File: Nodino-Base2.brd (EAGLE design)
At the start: 64.8 x 27.9 mm, 6 parts, among them CON1 NODINO-JTAGBASE, CON2 NODINO-JTAGBASE, IC5 AMS1117-3.3

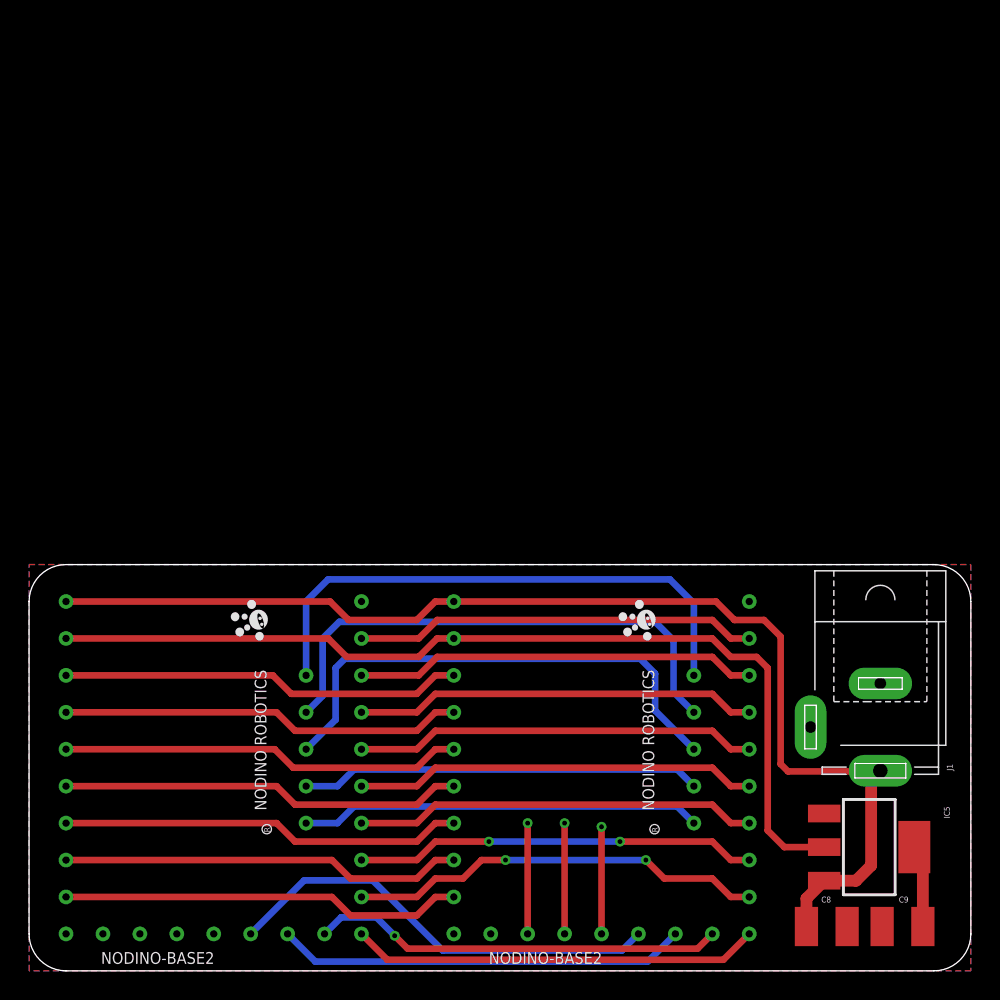
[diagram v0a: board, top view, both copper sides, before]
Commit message: final version
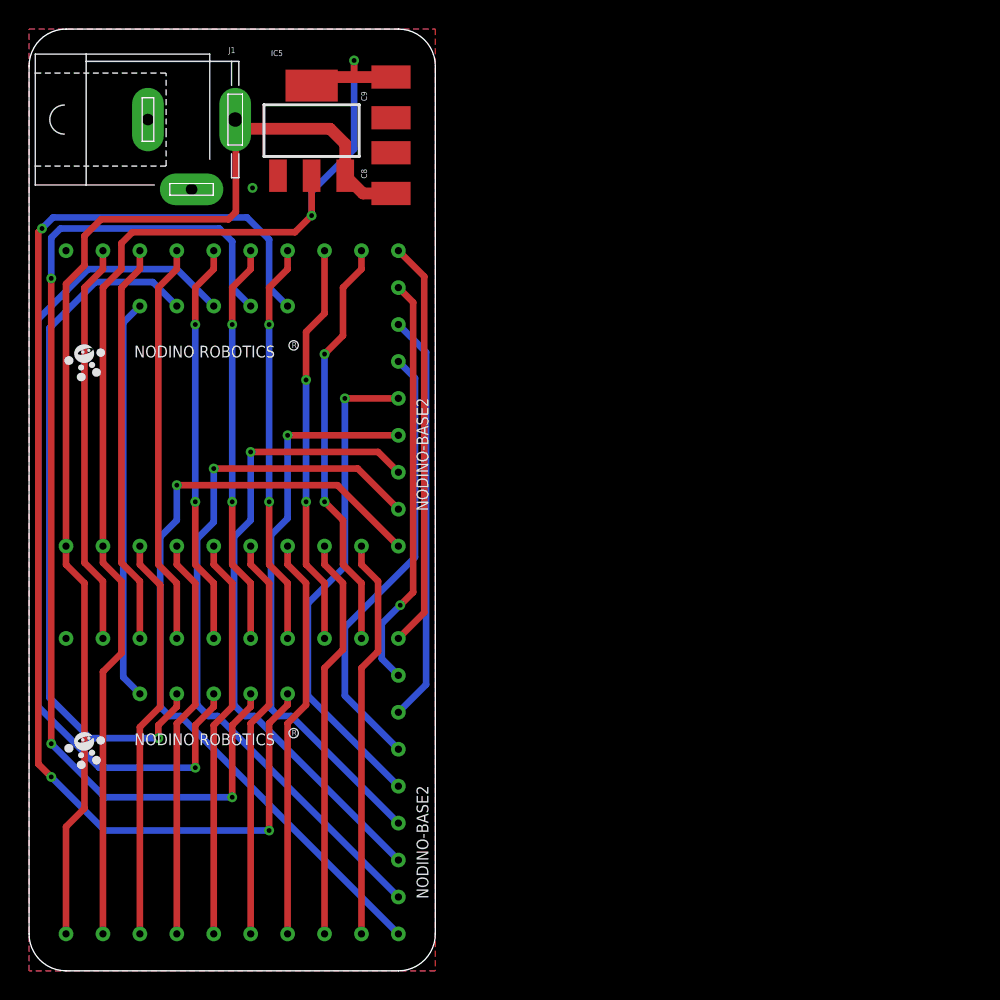
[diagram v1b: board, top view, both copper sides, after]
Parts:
- moved C9 67.0 mm to (24.9, 60.1), turned to 270 degrees
- moved J1 63.2 mm to (11.2, 58.5), turned to 0 degrees
- moved IC5 62.4 mm to (19.4, 57.8), turned to 0 degrees
- moved C8 59.9 mm to (24.9, 54.9), turned to 90 degrees
- moved CON2 35.9 mm to (14.0, 39.4), turned to 0 degrees
- moved CON1 1.80 mm to (14.0, 12.7), turned to 0 degrees
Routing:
- net JTCK: track 27.6 -> 86.3 mm, vias 0 -> 3
- net REF: track 0.00 -> 55.5 mm, vias 0 -> 1
- net A0: track 0.00 -> 49.9 mm, vias 0 -> 1
- net JTDI: track 27.6 -> 74.5 mm, vias 0 -> 3
- net A1: track 7.62 -> 44.3 mm
- net A2: track 7.62 -> 38.9 mm
- net A3: track 7.37 -> 34.0 mm
- net JTDO: track 35.4 -> 59.3 mm, vias 0 -> 1
- net +3V3: track 71.4 -> 84.4 mm, vias 0 -> 2
- net JTMS: track 36.2 -> 48.4 mm, vias 0 -> 1
- net JTRST: track 38.0 -> 27.6 mm
- net D4: vias 0 -> 2
- net D3: vias 0 -> 2
- net D2: vias 0 -> 2
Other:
- board size 64.8 x 27.9 mm -> 27.9 x 64.8 mm
